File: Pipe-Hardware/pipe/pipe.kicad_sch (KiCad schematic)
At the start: 12 parts, among them J1 Screw_Terminal_01x02, U1 ATmega32A-P, U2 MPU6050, U3 AT24C512B-PU25, U4 LLV, U5 AMS1117, U6 HC-5

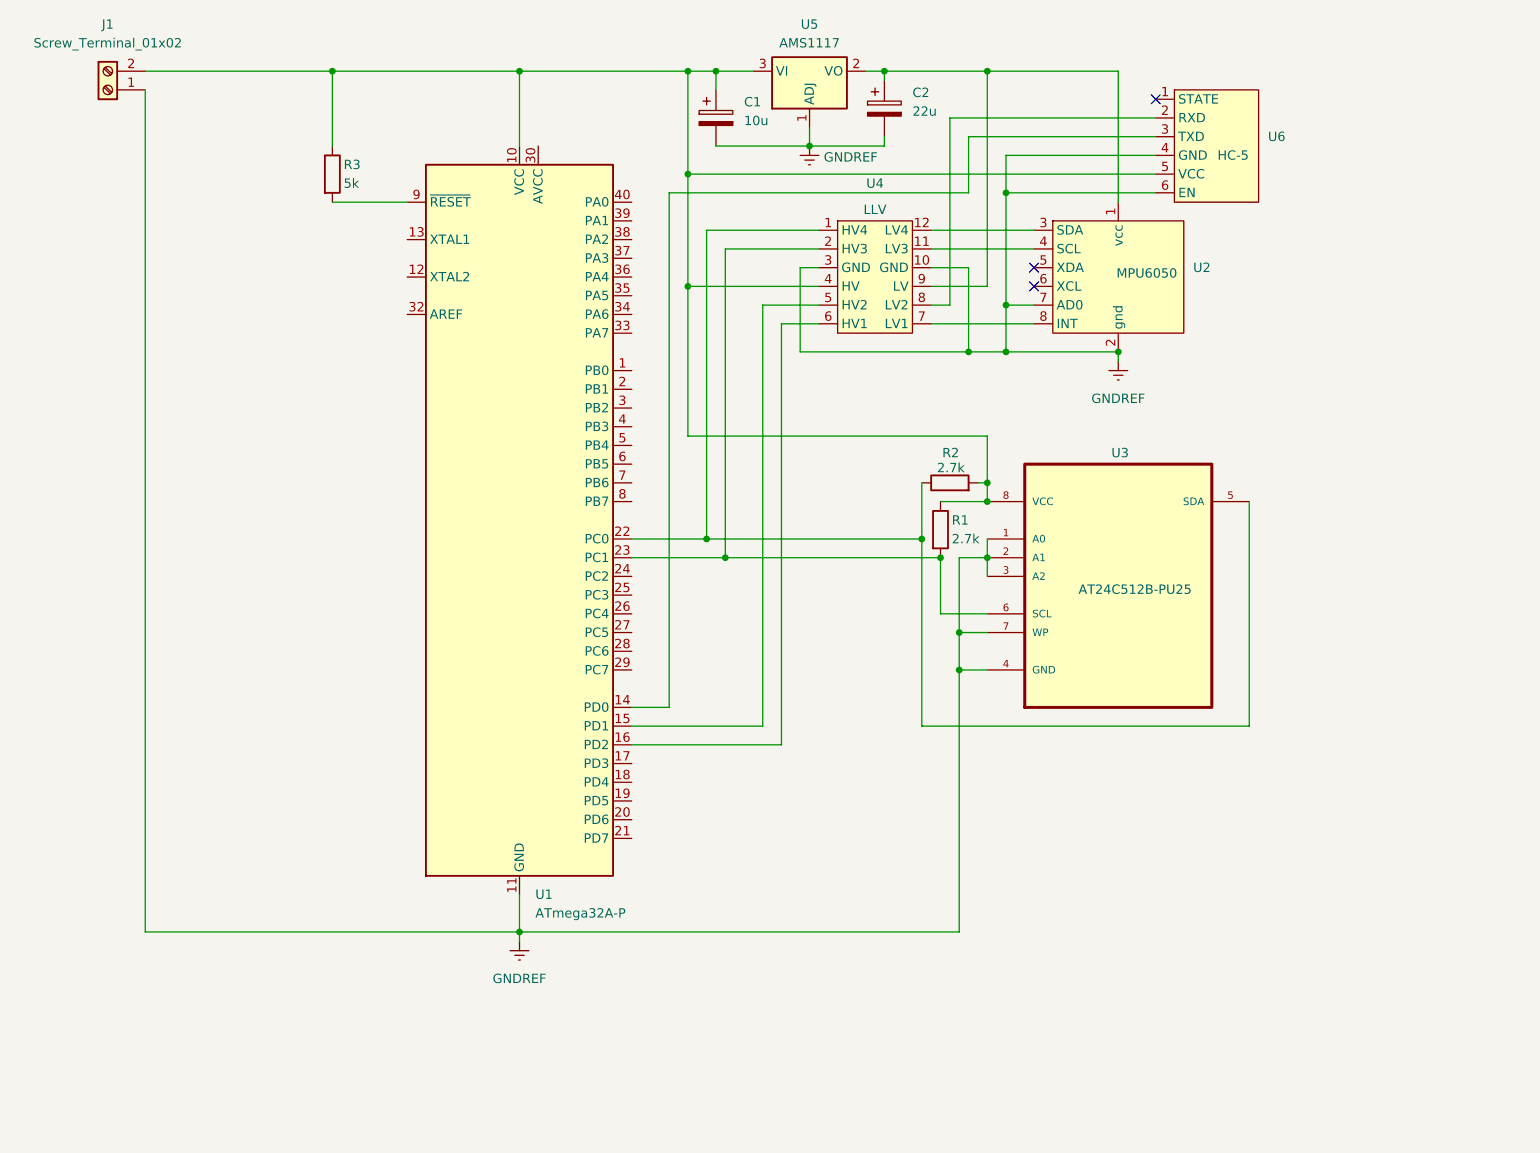
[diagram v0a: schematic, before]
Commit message: تعديل الإسطوانة
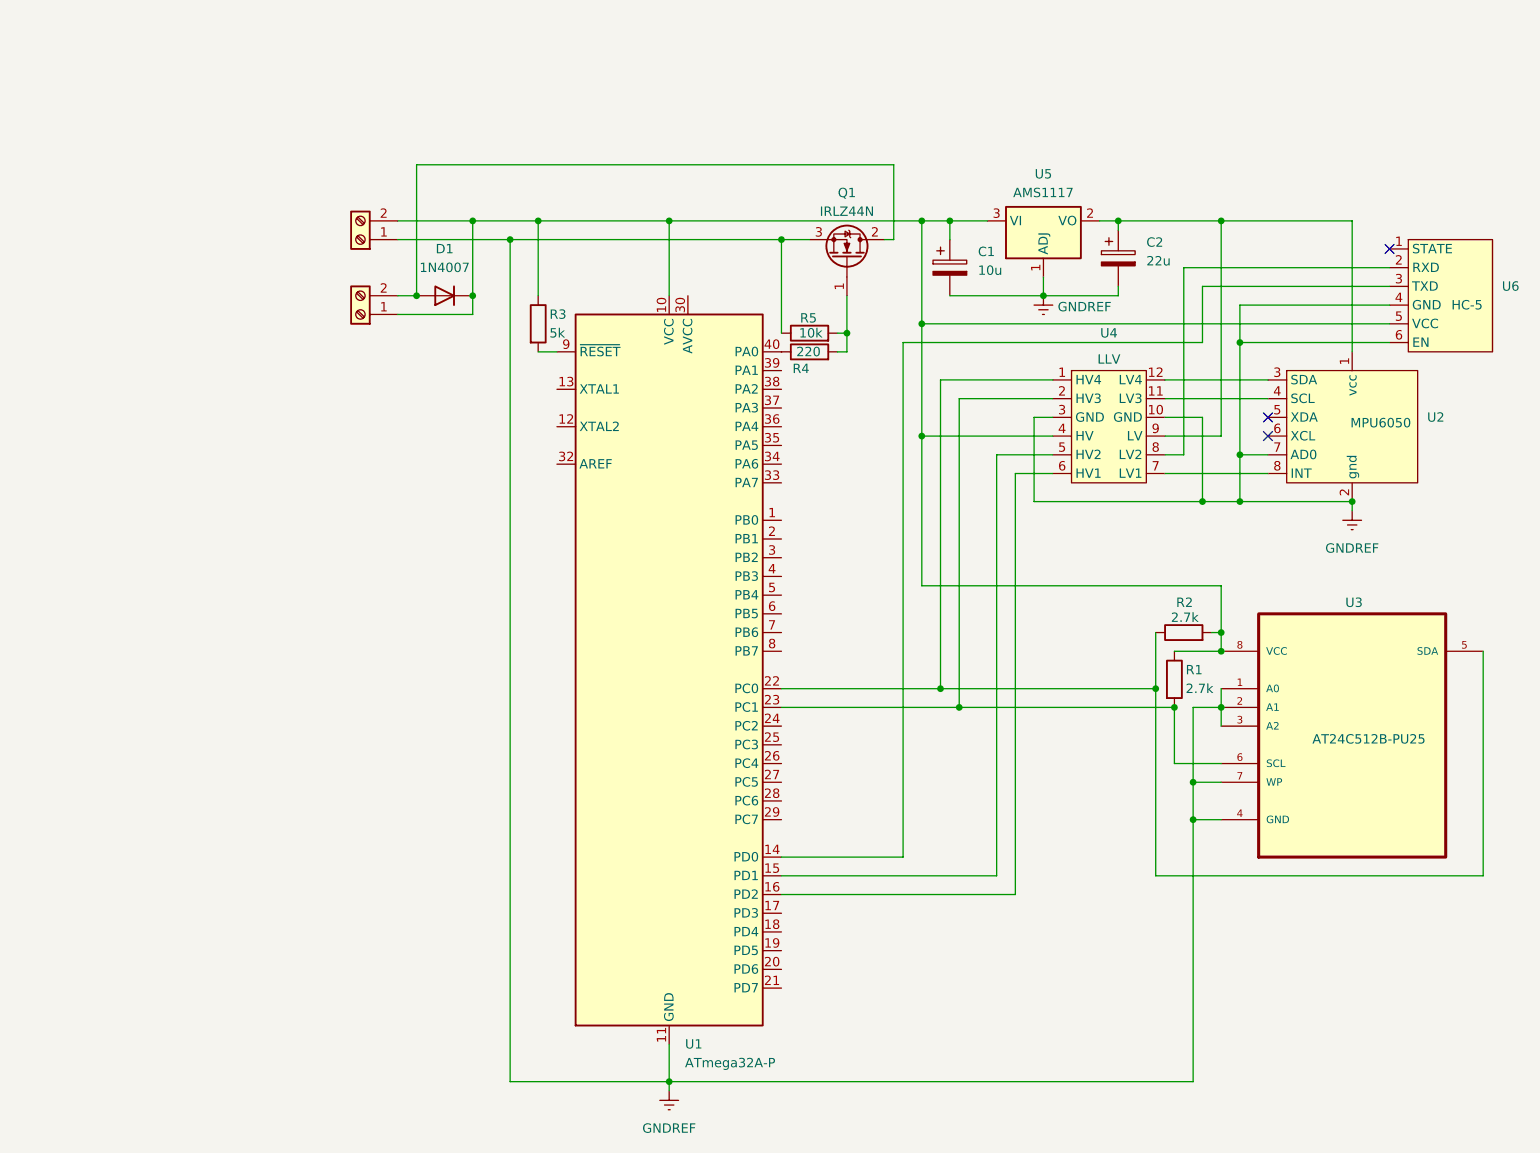
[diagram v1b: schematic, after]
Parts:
- added D1: 1N4007, Diode_THT:D_DO-41_SOD81_P10.16mm_Horizontal, symbol Diode:1N4007
- added J2: Screw_Terminal_01x02, TerminalBlock:TerminalBlock_MaiXu_MX126-5.0-02P_1x02_P5.00mm, symbol Connector:Screw_Terminal_01x02
- added Q1: IRLZ44N, Package_TO_SOT_THT:TO-220-3_Vertical, symbol Transistor_FET:IRLZ44N
- added R4: 220, Resistor_THT:R_Axial_DIN0204_L3.6mm_D1.6mm_P5.08mm_Horizontal, symbol Device:R
- added R5: 10k, Resistor_THT:R_Axial_DIN0204_L3.6mm_D1.6mm_P5.08mm_Horizontal, symbol Device:R
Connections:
- net GNDREF: now also Q1.3 (S), R5.1
- net at C1.1, J1.2 (Pin_2), R1.1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: now also D1.1 (K), J2.1 (Pin_1)
- net at U1.40 (PA0): now also R4.1
- new net: Q1.1 (G), R4.2, R5.2
- new net: D1.2 (A), J2.2 (Pin_2), Q1.2 (D)
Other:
- moved on the sheet: C1, C2, R1, R2, R3, U1, U2, U3, U4, U5, U6
